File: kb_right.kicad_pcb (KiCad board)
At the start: 2 copper layers, 208.8 x 117.5 mm, 175 parts, among them J1 10029449-001RLF, J2 Conn_01x03, J3 Conn_01x06, J4 Conn_01x08, J5 Conn_01x09, SW0 RotaryEncoder_Switch

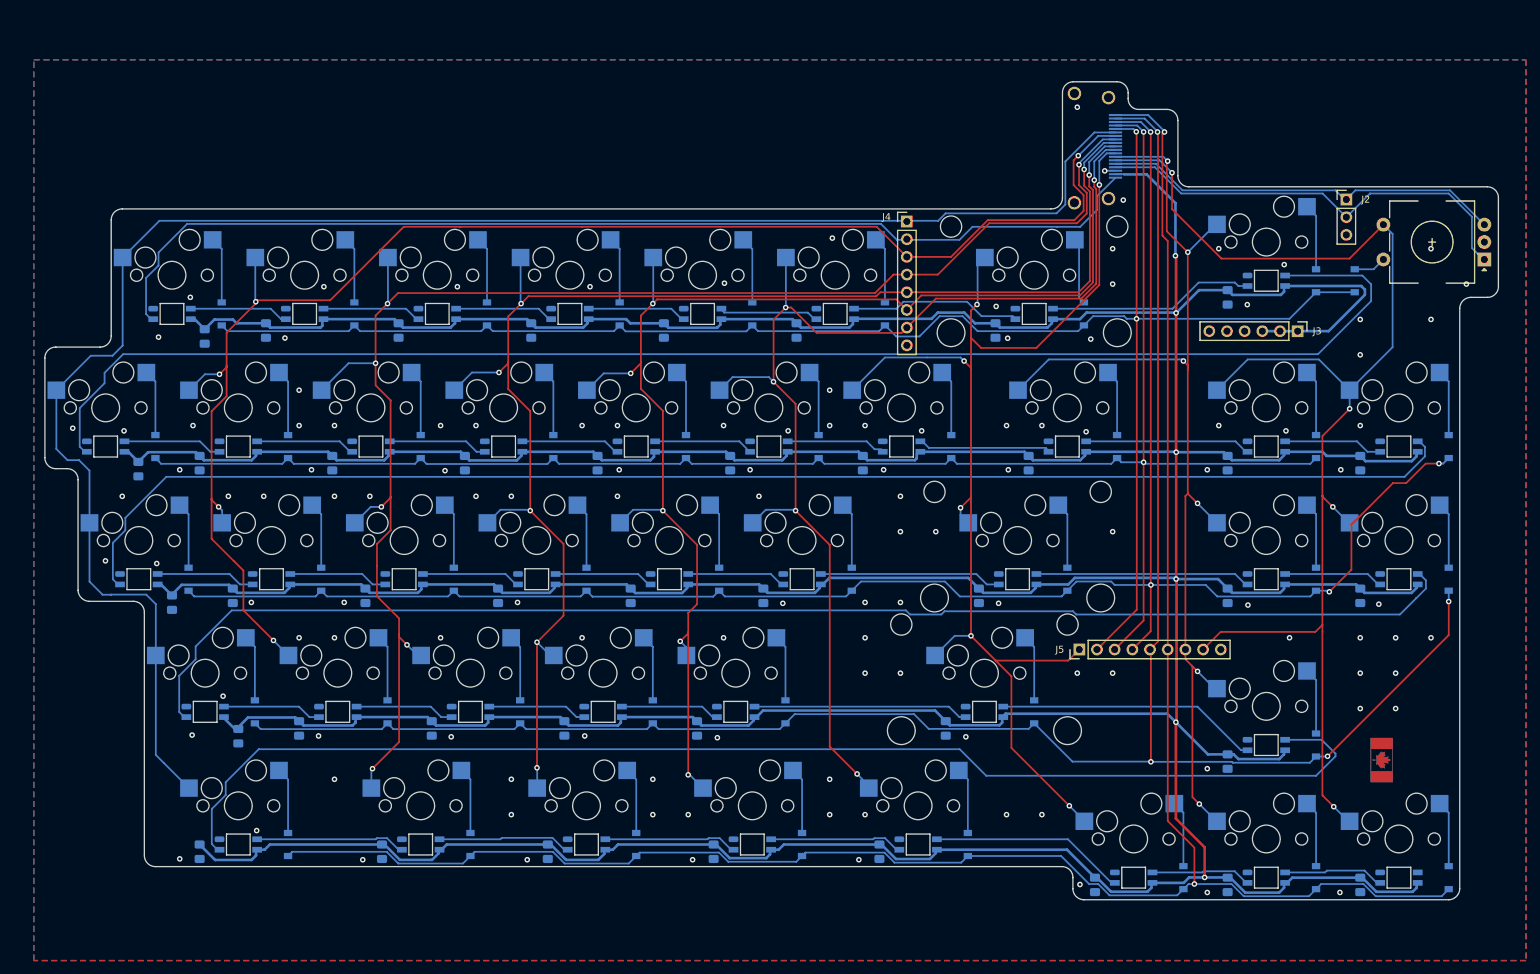
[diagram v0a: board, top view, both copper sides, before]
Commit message: added 1.75u right shift
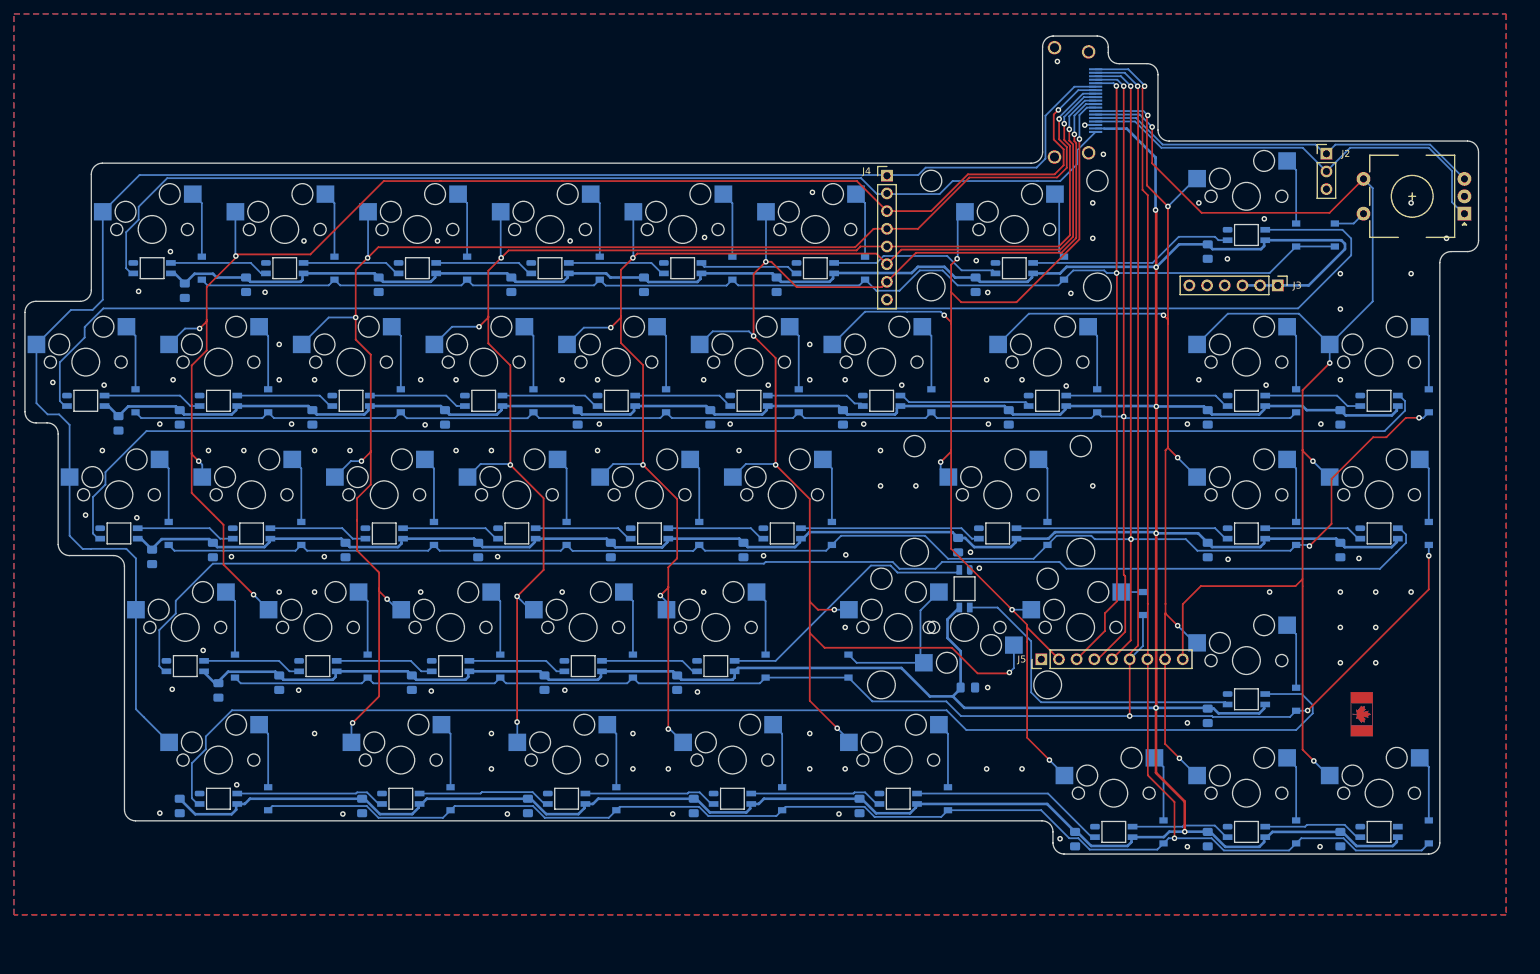
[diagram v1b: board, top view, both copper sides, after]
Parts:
- added D32_1: D_Small, Diode_SMD:D_SOD-123, B.Cu at (197.9, 110.9)
- added MX32_1: MX-NoLED, MX_Only:MXOnly-1.75U-Hotswap, F.Cu at (162.7, 114.3)
- added MX32_2: MX-NoLED, MX_Only:MXOnly-1U-Hotswap, F.Cu at (188.9, 114.3)
- C101, C102, C103, C104, C105, C106, C107, C108, C109, C110, C111, C112, C113, C114, C115, C116, C117, C118, C119, C120, C121, C122, C123, C124, C125, C126, C127, C128, C129, C130, C131, C132, C133, C134, C135, C136, C137, C138, C139, C140, C141, C142: value C_Small -> 0.1uF
- MX32: footprint MX_Only:MXOnly-2.75U-Hotswap -> MX_Only:MXOnly-2.75U-Hotswap-ReversedStabilizers
- moved D32 27.5 mm to (155.6, 119.9)
- moved D133 17.9 mm to (172.2, 108.7), turned to 90 degrees
- moved C125 7.86 mm to (171.3, 102.5)
- moved D141 7.17 mm to (212.7, 143.7)
- moved D40 7.17 mm to (200.8, 143.7)
- moved D42 7.17 mm to (238.9, 143.7)
- moved D140 7.17 mm to (193.7, 143.7)
- moved D142 7.17 mm to (231.8, 143.7)
- moved D41 7.17 mm to (219.9, 143.7)
- moved D114 7.17 mm to (141.3, 81.8)
- moved D117 7.17 mm to (212.7, 81.8)
- moved D13 7.17 mm to (129.4, 81.8)
- moved D15 7.17 mm to (167.5, 81.8)
- moved D16 7.17 mm to (191.3, 81.8)
- moved D26 7.17 mm to (238.9, 81.8)
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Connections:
- J5 pad 1: /COL6 -> GND
- J5 pad 2: /ROW5 -> /COL6
- J5 pad 3: /ROW6 -> /ROW5
- J5 pad 4: /ROW7 -> /ROW6
- J5 pad 5: /ROW8 -> /ROW7
- J5 pad 6: /ROW9 -> /ROW8
- J5 pad 7: /COL7 -> /ROW9
- J5 pad 8: /COL8 -> /COL7
- J5 pad 9: GND -> /COL8
- MX32 pad 1: /COL6 -> /COL5
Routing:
- net /COL5: track 168.8 -> 210.3 mm, vias 5 -> 7
- net Net-(MX32-Pad2): track 9.53 -> 22.8 mm
- net +5V: track 1059.3 -> 1072.0 mm
- net /COL6: track 175.6 -> 166.0 mm
- net Net-(D133-Pad2): track 38.0 -> 47.1 mm
- net /ROW7: track 280.9 -> 289.9 mm
- net /ROW6: track 252.7 -> 261.1 mm
- net /COL8: track 188.4 -> 196.4 mm
- net /ROW5: track 251.4 -> 259.4 mm
- net Net-(D132-Pad2): track 31.2 -> 38.5 mm
- net /ROW8: track 290.1 -> 295.5 mm
- net Net-(D32_1-Pad2): track 0.00 -> 3.11 mm
- net /COL7: track 149.7 -> 151.2 mm
- net Net-(D134-Pad2): track 183.9 -> 182.7 mm
- net Net-(D127-Pad2): track 195.8 -> 196.5 mm
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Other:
- outline, holes or cut-outs redrawn
